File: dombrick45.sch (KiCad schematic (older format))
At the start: 5 parts

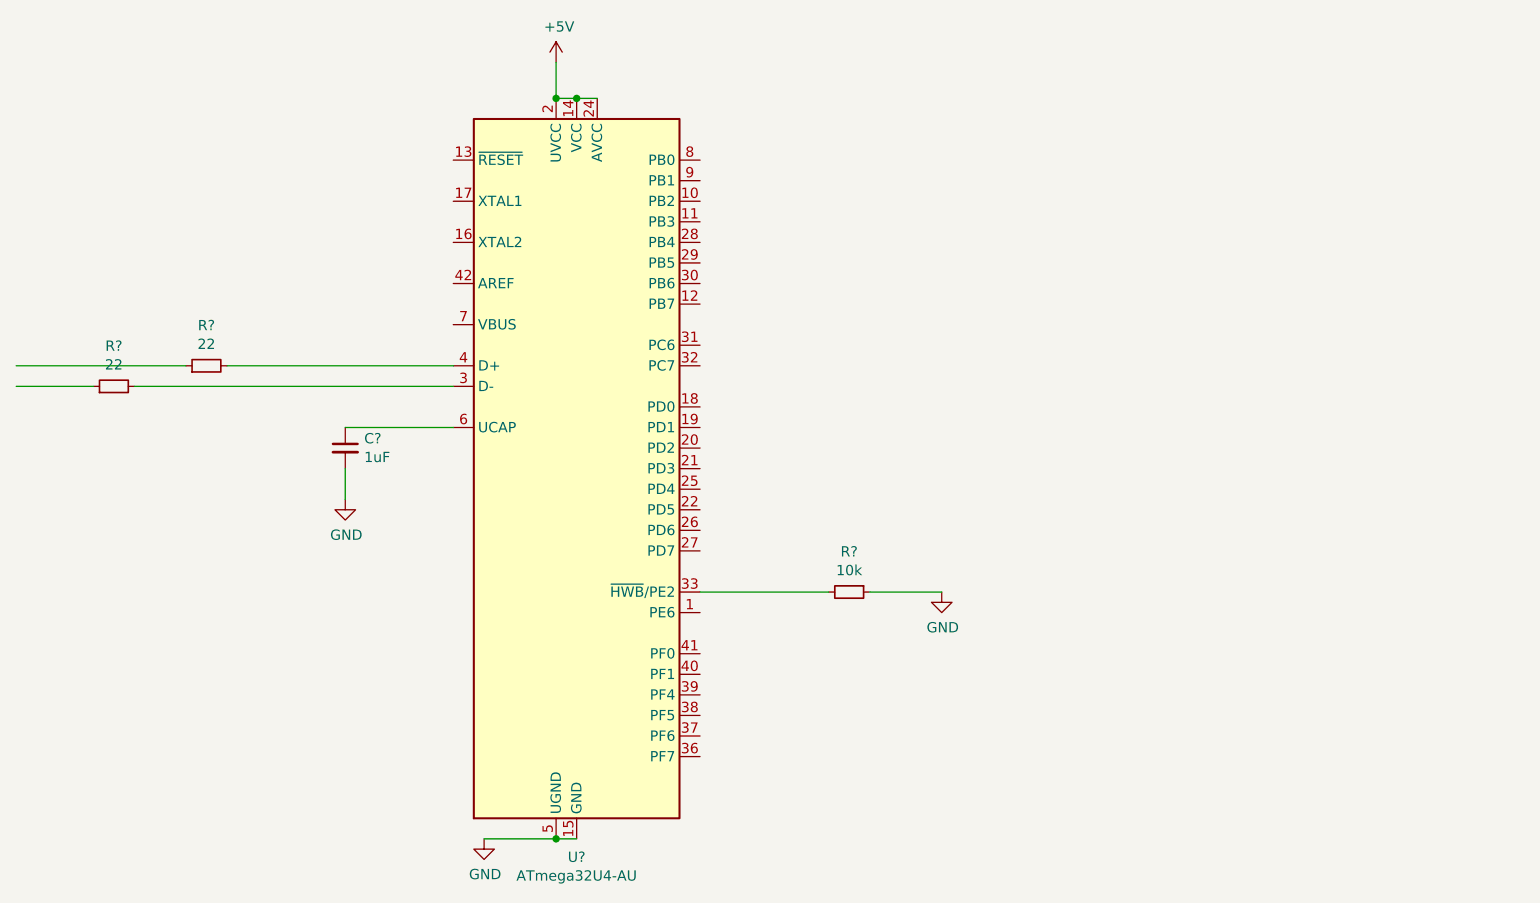
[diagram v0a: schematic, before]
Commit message: 2019-10-04
2019-10-04 ai10さんブログの演習途中
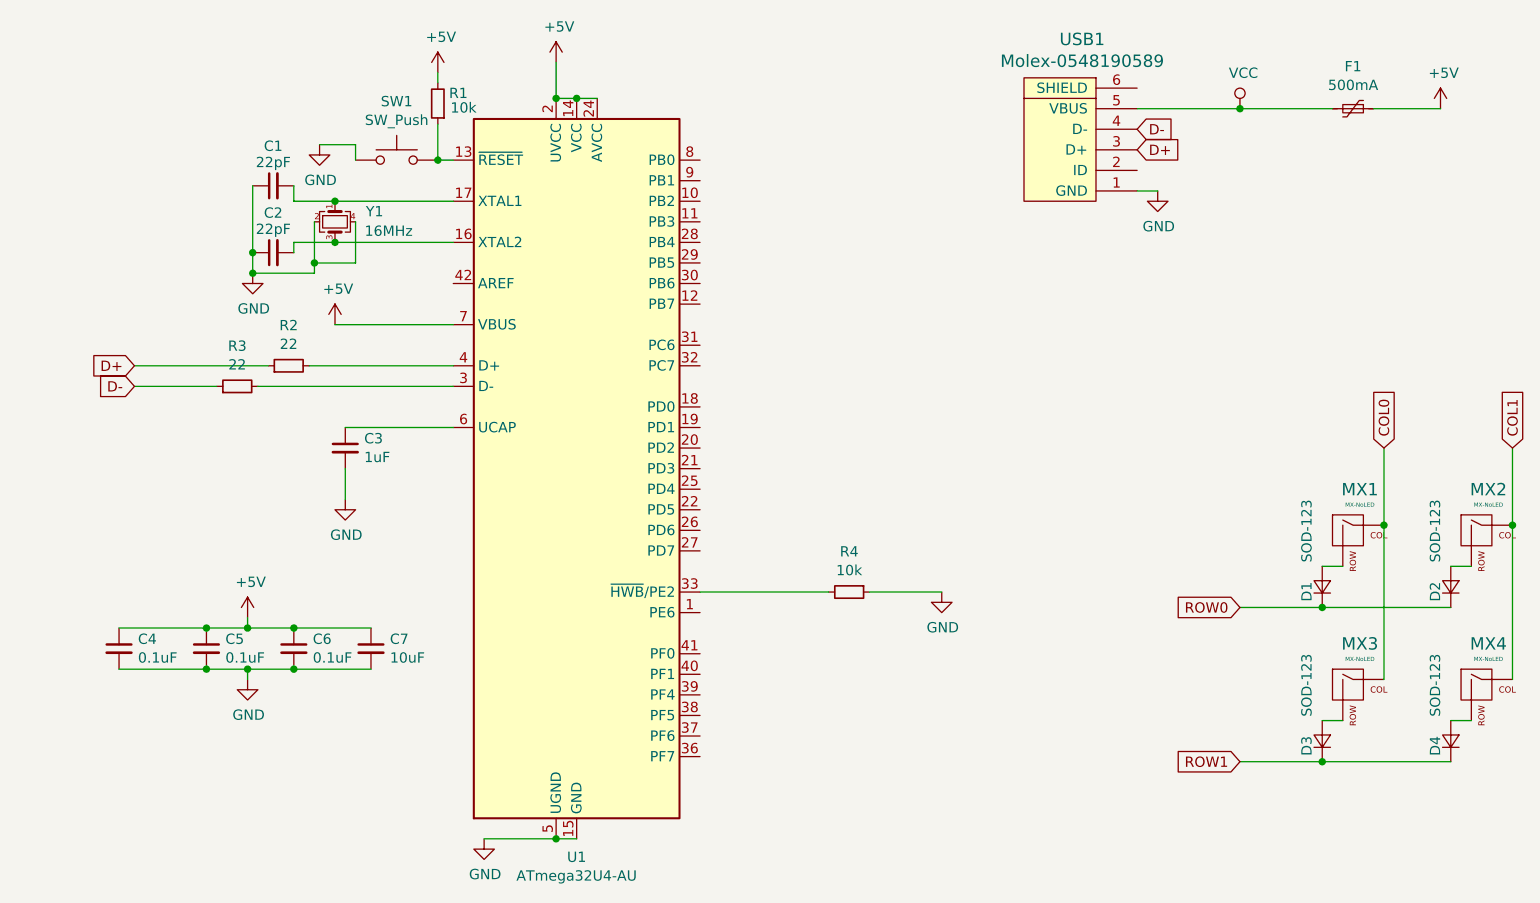
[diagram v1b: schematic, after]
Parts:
- added C1, C2: 22pF, Capacitor_SMD:C_0805_2012Metric, symbol Device:C_Small
- added C4, C5, C6: 0.1uF, Capacitor_SMD:C_0805_2012Metric, symbol Device:C_Small
- added C7: 10uF, Capacitor_SMD:C_0805_2012Metric, symbol Device:C_Small
- added D1, D2, D3, D4: SOD-123, Diode_SMD:D_SOD-123, symbol Device:D_Small
- added F1: 500mA, Fuse:Fuse_1206_3216Metric, symbol Device:Polyfuse_Small
- added MX1, MX2, MX3, MX4: MX-NoLED, MX_Alps_Hybrid:MX-1U-NoLED, symbol MX_Alps_Hybrid:MX-NoLED
- added R1: 10k, Resistor_SMD:R_0805_2012Metric, symbol Device:R_Small
- added SW1: SW_Push, symbol Switch:SW_Push
- added USB1: Molex-0548190589, symbol random-keyboard-parts:Molex-0548190589
- added Y1: 16MHz, symbol Device:Crystal_GND24_Small
- C3: renamed from C?; footprint (none) -> Capacitor_SMD:C_0805_2012Metric
- R2, R3, R4: renamed from R?; footprint (none) -> Resistor_SMD:R_0805_2012Metric
- gave numbers to parts that had none: 1
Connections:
- net labels added: COL0, COL1, D+, D-, ROW0, ROW1, VCC
- wire segments 13 -> 58
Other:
- moved on the sheet: R2, R3

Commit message: 2019-10-06
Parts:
- C1, C2, C3, C4, C5, C6, C7: footprint Capacitor_SMD:C_0805_2012Metric -> Capacitor_SMD:C_0805_2012Metric_Pad1.15x1.40mm_HandSolder
- SW1: footprint (none) -> random-keyboard-parts:SKQG-1155865
- USB1: footprint (none) -> random-keyboard-parts:Molex-0548190589
- Y1: footprint (none) -> Crystal:Crystal_SMD_3225-4Pin_3.2x2.5mm
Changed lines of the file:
@@
 F 0 "C3" H 2992 3271 50  0000 L CNN
 F 1 "1uF" H 2992 3180 50  0000 L CNN
-F 2 "Capacitor_SMD:C_0805_2012Metric" H 2900 3225 50  0001 C CNN
+F 2 "Capacitor_SMD:C_0805_2012Metric_Pad1.15x1.40mm_HandSolder" H 2900 3225 50  0001 C CNN
 F 3 "~" H 2900 3225 50  0001 C CNN
 	1    2900 3225
@@
 F 0 "C4" H 1892 4246 50  0000 L CNN
 F 1 "0.1uF" H 1892 4155 50  0000 L CNN
-F 2 "Capacitor_SMD:C_0805_2012Metric" H 1800 4200 50  0001 C CNN
+F 2 "Capacitor_SMD:C_0805_2012Metric_Pad1.15x1.40mm_HandSolder" H 1800 4200 50  0001 C CNN
 F 3 "~" H 1800 4200 50  0001 C CNN
 	1    1800 4200
@@
 F 0 "C5" H 2317 4246 50  0000 L CNN
 F 1 "0.1uF" H 2317 4155 50  0000 L CNN
-F 2 "Capacitor_SMD:C_0805_2012Metric" H 2225 4200 50  0001 C CNN
+F 2 "Capacitor_SMD:C_0805_2012Metric_Pad1.15x1.40mm_HandSolder" H 2225 4200 50  0001 C CNN
 F 3 "~" H 2225 4200 50  0001 C CNN
 	1    2225 4200
@@
 F 0 "C6" H 2742 4246 50  0000 L CNN
 F 1 "0.1uF" H 2742 4155 50  0000 L CNN
-F 2 "Capacitor_SMD:C_0805_2012Metric" H 2650 4200 50  0001 C CNN
+F 2 "Capacitor_SMD:C_0805_2012Metric_Pad1.15x1.40mm_HandSolder" H 2650 4200 50  0001 C CNN
 F 3 "~" H 2650 4200 50  0001 C CNN
 	1    2650 4200
@@
 F 0 "C7" H 3117 4246 50  0000 L CNN
 F 1 "10uF" H 3117 4155 50  0000 L CNN
-F 2 "Capacitor_SMD:C_0805_2012Metric" H 3025 4200 50  0001 C CNN
+F 2 "Capacitor_SMD:C_0805_2012Metric_Pad1.15x1.40mm_HandSolder" H 3025 4200 50  0001 C CNN
 F 3 "~" H 3025 4200 50  0001 C CNN
 	1    3025 4200
@@
 F 0 "SW1" H 3150 2110 50  0000 C CNN
 F 1 "SW_Push" H 3150 2019 50  0000 C CNN
-F 2 "" H 3150 2025 50  0001 C CNN
+F 2 "random-keyboard-parts:SKQG-1155865" H 3150 2025 50  0001 C CNN
 F 3 "~" H 3150 2025 50  0001 C CNN
 	1    3150 1825
@@
 F 0 "C2" V 2743 2275 50  0000 C CNN
 F 1 "22pF" V 2664 2275 50  0000 C CNN
-F 2 "Capacitor_SMD:C_0805_2012Metric" H 2550 2275 50  0001 C CNN
+F 2 "Capacitor_SMD:C_0805_2012Metric_Pad1.15x1.40mm_HandSolder" H 2550 2275 50  0001 C CNN
 F 3 "~" H 2550 2275 50  0001 C CNN
 	1    2550 2275
@@
 F 0 "C1" V 2743 1950 50  0000 C CNN
 F 1 "22pF" V 2664 1950 50  0000 C CNN
-F 2 "Capacitor_SMD:C_0805_2012Metric" H 2550 1950 50  0001 C CNN
+F 2 "Capacitor_SMD:C_0805_2012Metric_Pad1.15x1.40mm_HandSolder" H 2550 1950 50  0001 C CNN
 F 3 "~" H 2550 1950 50  0001 C CNN
 	1    2550 1950
@@
 F 0 "Y1" V 2800 2275 50  0000 L CNN
 F 1 "16MHz" V 2895 2269 50  0000 L CNN
-F 2 "" H 2850 2125 50  0001 C CNN
+F 2 "Crystal:Crystal_SMD_3225-4Pin_3.2x2.5mm" H 2850 2125 50  0001 C CNN
 F 3 "~" H 2850 2125 50  0001 C CNN
 	1    2850 2125
@@
 F 0 "USB1" V 6987 1742 60  0000 C CNN
 F 1 "Molex-0548190589" V 6881 1742 60  0000 C CNN
-F 2 "" H 6450 1775 60  0001 C CNN
+F 2 "random-keyboard-parts:Molex-0548190589" H 6450 1775 60  0001 C CNN
 F 3 "" H 6450 1775 60  0001 C CNN
 	1    6450 1775

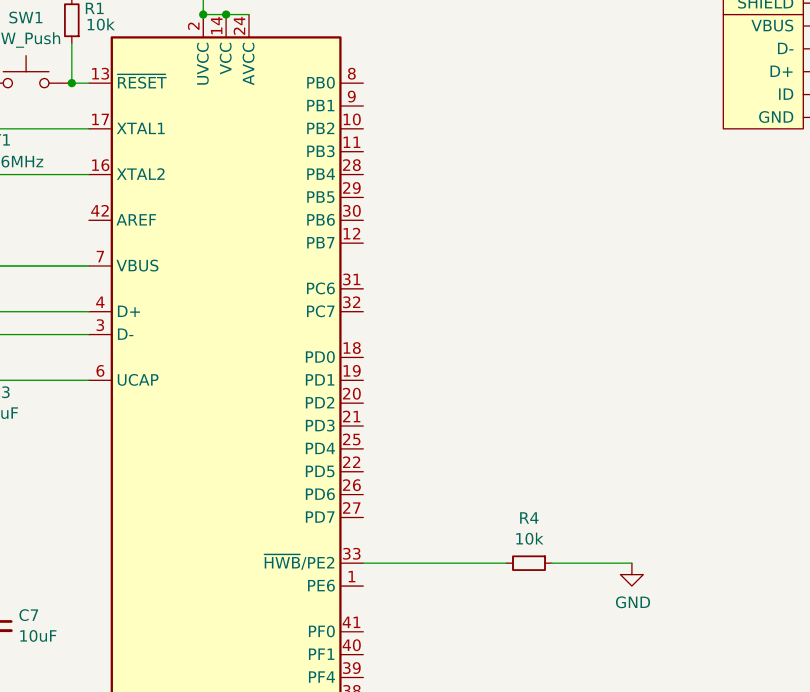
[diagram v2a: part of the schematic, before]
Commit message: 2019-10-06 tutorial
hobo kansei
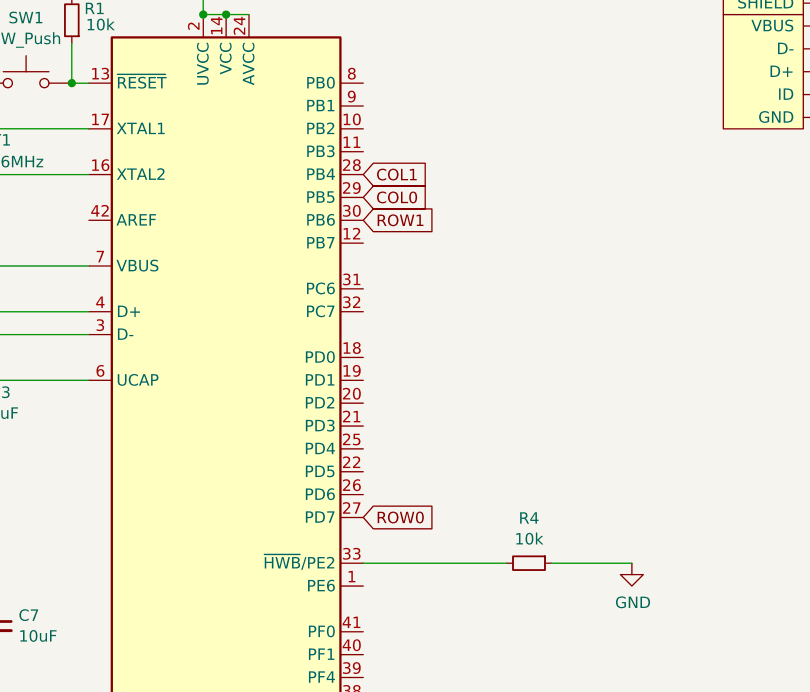
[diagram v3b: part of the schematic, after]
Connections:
- net COL0: now also U1.29 (PB5)
- net COL1: now also U1.28 (PB4)
- net ROW0: now also U1.27 (PD7)
- net ROW1: now also U1.30 (PB6)
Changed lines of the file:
@@
 $EndDescr
-$Comp
-L MCU_Microchip_ATmega:ATmega32U4-AU U1
-U 1 1 5D9215A6
-P 4025 3325
-F 0 "U1" H 4025 1436 50  0000 C CNN
-F 1 "ATmega32U4-AU" H 4025 1345 50  0000 C CNN
-F 2 "Package_QFP:TQFP-44_10x10mm_P0.8mm" H 4025 3325 50  0001 C CIN
-F 3 "http://ww1.microchip.com/downloads/en/DeviceDoc/Atmel-7766-8-bit-AVR-ATmega16U4-32U4_Datasheet.pdf" H 4025 3325 50  0001 C CNN
-	1    4025 3325
-	1    0    0    -1
-$EndComp
 $Comp
 L power:+5V #PWR0101
@@
 Text GLabel 7250 4750 0    50   Input ~ 0
 ROW1
+$Comp
+L MCU_Microchip_ATmega:ATmega32U4-AU U1
+U 1 1 5D9215A6
+P 4025 3325
+F 0 "U1" H 4025 1436 50  0000 C CNN
+F 1 "ATmega32U4-AU" H 4025 1345 50  0000 C CNN
+F 2 "Package_QFP:TQFP-44_10x10mm_P0.8mm" H 4025 3325 50  0001 C CIN
+F 3 "http://ww1.microchip.com/downloads/en/DeviceDoc/Atmel-7766-8-bit-AVR-ATmega16U4-32U4_Datasheet.pdf" H 4025 3325 50  0001 C CNN
+	1    4025 3325
+	1    0    0    -1
+$EndComp
+Text GLabel 4625 3725 2    50   Input ~ 0
+ROW0
+Text GLabel 4625 2425 2    50   Input ~ 0
+ROW1
+Text GLabel 4625 2325 2    50   Input ~ 0
+COL0
+Text GLabel 4625 2225 2    50   Input ~ 0
+COL1
 $EndSCHEMATC
